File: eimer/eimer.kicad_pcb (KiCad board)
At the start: 2 copper layers, 72 x 72 mm, 71 parts, among them J3 Conn_01x03, J4 USB_C_Receptacle_USB2.0_14P, SW1 SW_Push, SW2 SW_Push, U1 RP2040, U2 MCP1700x-330xxTT, U3 TPS61221DCK, U4 W25Q16JVUXIQ TR, U5 LIS2DW12, Y1 12 MHz

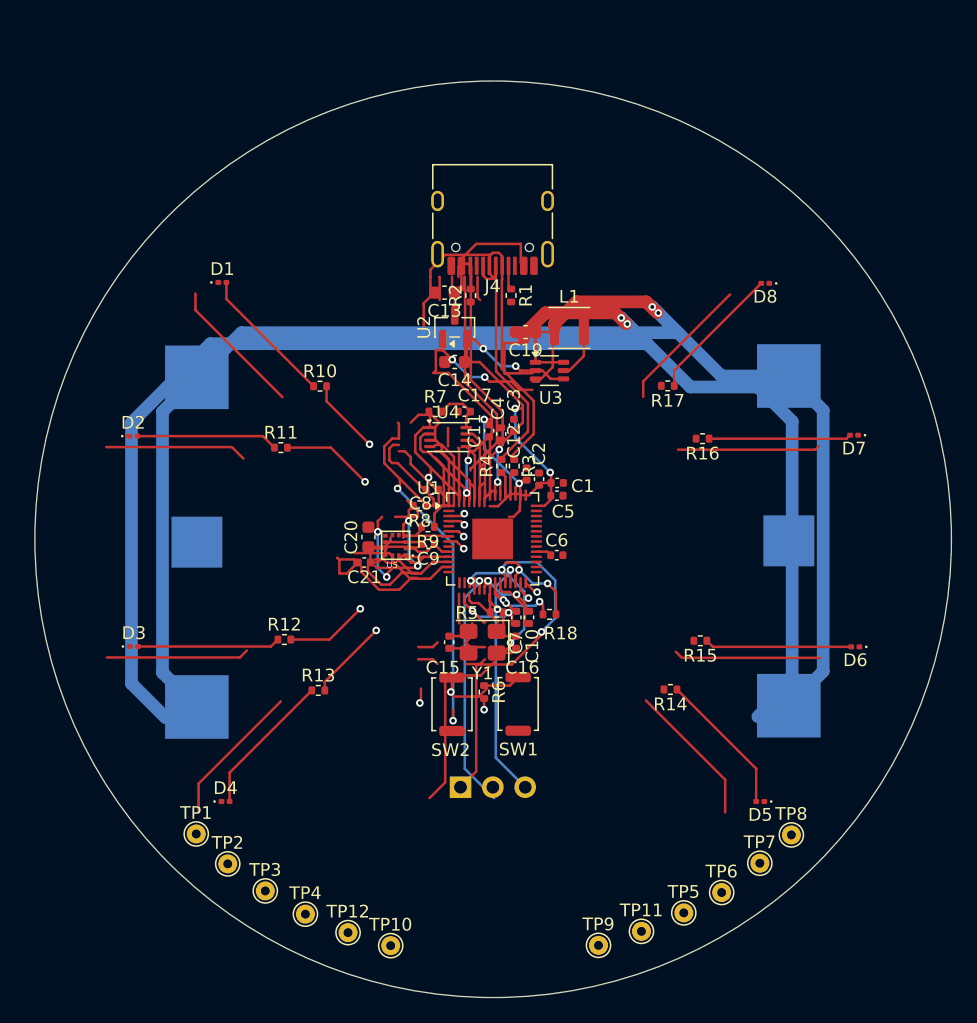
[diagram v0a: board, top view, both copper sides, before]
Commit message: revert
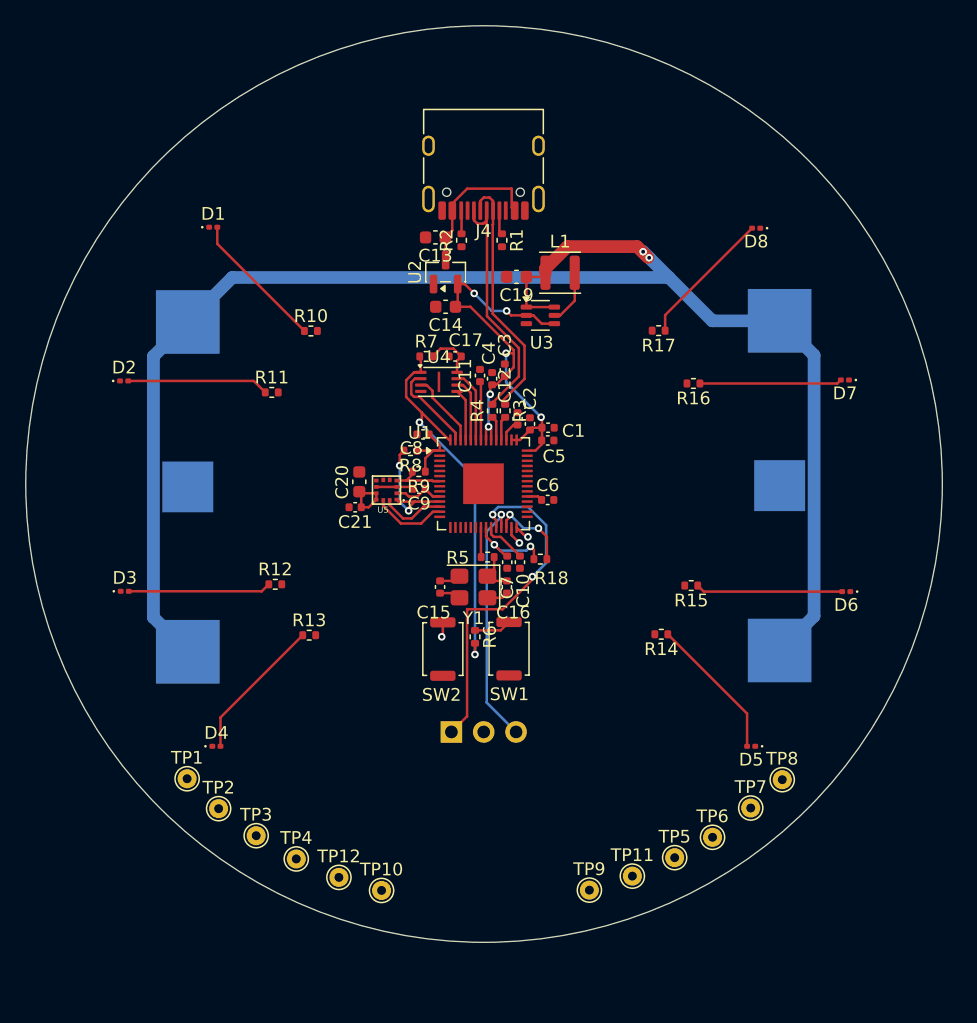
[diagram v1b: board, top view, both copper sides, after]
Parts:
- moved J4 4.40 mm to (73.8, 63.5)
- moved C20 4.40 mm to (64.1, 88.9)
- moved C8 4.40 mm to (69.1, 85.1)
- moved C9 4.40 mm to (68.8, 89.4)
- moved D6 4.40 mm to (102.3, 97.5)
- moved R17 4.40 mm to (87.6, 77.0)
- moved R7 4.40 mm to (69.3, 79.0)
- moved TP10 4.40 mm to (65.8, 121.0)
- moved TP11 4.40 mm to (85.5, 119.8)
- moved TP6 4.40 mm to (91.8, 116.8)
- moved TP7 4.40 mm to (94.8, 114.5)
- moved TP9 4.40 mm to (82.1, 121.0)
- moved U1 4.40 mm to (73.8, 89.0)
- moved U4 4.40 mm to (70.3, 81.0)
- moved C21 4.40 mm to (63.7, 90.9)
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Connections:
- R10 pad 2: GPIO1 -> GPIO11
- R11 pad 2: GPIO2 -> GPIO12
- R12 pad 2: GPIO4 -> GPIO13
- R13 pad 2: GPIO6 -> unconnected-(R13-Pad2)
- R14 pad 2: GPIO26/ADC0 -> GPIO15
- R15 pad 2: GPIO27/ADC1 -> GPIO16
- R16 pad 2: GPIO28/ADC2 -> GPIO17
- R17 pad 2: GPIO29/ADC3 -> GPIO18
- TP1 pad 1: unconnected-(TP1-Pad1) -> GPIO26/ADC0
- TP2 pad 1: unconnected-(TP2-Pad1) -> GPIO27/ADC1
- TP3 pad 1: unconnected-(TP3-Pad1) -> GPIO28/ADC2
- TP4 pad 1: unconnected-(TP4-Pad1) -> GPIO29/ADC3
- TP5 pad 1: unconnected-(TP5-Pad1) -> GPIO20
- TP6 pad 1: unconnected-(TP6-Pad1) -> GPIO22
- TP7 pad 1: unconnected-(TP7-Pad1) -> GPIO23
- TP8 pad 1: unconnected-(TP8-Pad1) -> GPIO24
- U1 pad 14: unconnected-(U1-GPIO11-Pad14) -> GPIO11
- U1 pad 15: unconnected-(U1-GPIO12-Pad15) -> GPIO12
- U1 pad 16: unconnected-(U1-GPIO13-Pad16) -> GPIO13
- U1 pad 17: unconnected-(U1-GPIO14-Pad17) -> GPIO14
- U1 pad 18: unconnected-(U1-GPIO15-Pad18) -> GPIO15
- U1 pad 27: unconnected-(U1-GPIO16-Pad27) -> GPIO16
- U1 pad 28: unconnected-(U1-GPIO17-Pad28) -> GPIO17
- U1 pad 29: unconnected-(U1-GPIO18-Pad29) -> GPIO18
- U1 pad 3: GPIO1 -> unconnected-(U1-GPIO1-Pad3)
- U1 pad 31: unconnected-(U1-GPIO20-Pad31) -> GPIO20
- U1 pad 34: unconnected-(U1-GPIO22-Pad34) -> GPIO22
- U1 pad 35: unconnected-(U1-GPIO23-Pad35) -> GPIO23
- U1 pad 36: unconnected-(U1-GPIO24-Pad36) -> GPIO24
- U1 pad 4: GPIO2 -> unconnected-(U1-GPIO2-Pad4)
- U1 pad 6: GPIO4 -> unconnected-(U1-GPIO4-Pad6)
- U1 pad 8: GPIO6 -> unconnected-(U1-GPIO6-Pad8)
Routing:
- net Net-(BT1-+): track 248.4 -> 124.2 mm, vias 4 -> 2
- net +3.3V: track 130.5 -> 65.9 mm, vias 16 -> 8
- net SWCLK: track 54.5 -> 27.2 mm, vias 4 -> 2
- net USB_D+: track 39.8 -> 19.9 mm
- net USB_D-: track 39.7 -> 19.8 mm
- net SWDIO: track 39.0 -> 19.5 mm, vias 2 -> 1
- net VBUS: track 23.3 -> 11.7 mm
- net Net-(D6-A): track 23.1 -> 11.5 mm
- net Net-(D4-A): track 22.8 -> 11.4 mm
- net Net-(D5-A): track 22.8 -> 11.4 mm
- net Net-(D3-A): track 22.4 -> 11.2 mm
- net Net-(D7-A): track 22.4 -> 11.2 mm
- net Net-(D2-A): track 22.3 -> 11.1 mm
- net Net-(D1-A): track 22.0 -> 11.0 mm
- net Net-(D8-A): track 21.8 -> 10.9 mm
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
